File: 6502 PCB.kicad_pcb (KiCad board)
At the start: 2 copper layers, 25 parts, among them SW1 RESET, SW2 SW_Push, SW3 SW_Push, SW4 SW_Push, SW5 SW_Push, SW6 SW_Push, U1 W65C02S, U2 28C256, U3 62256, U4 W65C22, U5 74HC00, X1 1MHz

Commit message: bumb
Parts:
- DS1: footprint Display:HY1602E -> Display:WC1602A
- moved DS1 220.6 mm to (27.9, 87.9)
- moved U2 90.1 mm to (22.9, 53.3), turned to 90 degrees
- moved SW4 69.8 mm to (147.3, 104.1)
- moved SW1 68.2 mm to (27.9, 25.4)
- moved X1 65.9 mm to (63.5, 27.9)
- moved C4 64.3 mm to (125.5, 37.9)
- moved C2 64.3 mm to (125.5, 28.2)
- moved C3 64.3 mm to (125.5, 33.0)
- moved R1 64.3 mm to (130.1, 29.8)
- moved R2 64.3 mm to (130.1, 31.6)
- moved R3 64.3 mm to (130.1, 33.3)
- moved R4 64.3 mm to (130.1, 35.1)
- moved R5 64.3 mm to (130.1, 36.8)
- moved R6 64.3 mm to (130.1, 38.6)
- moved R7 64.3 mm to (130.1, 40.3)
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
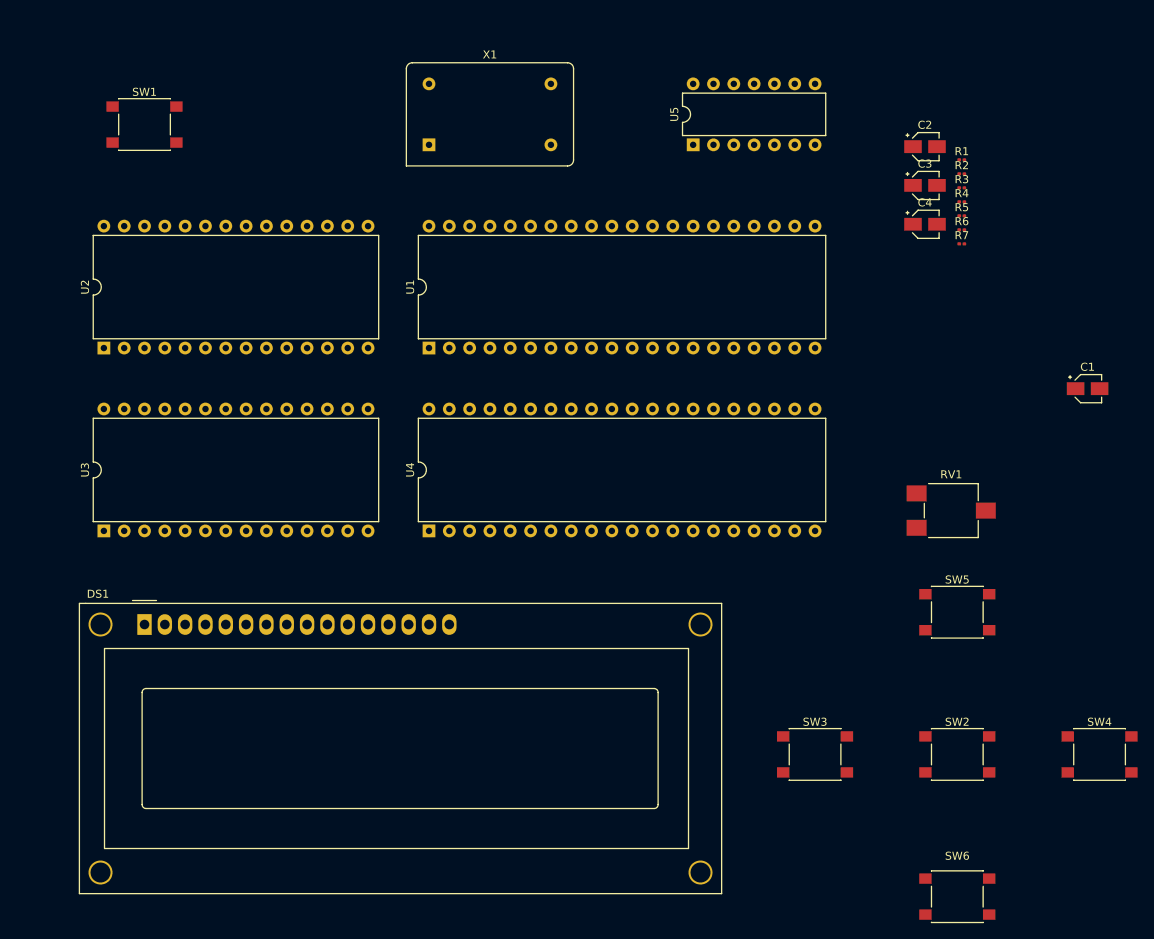
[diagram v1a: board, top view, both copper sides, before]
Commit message: Add files via upload
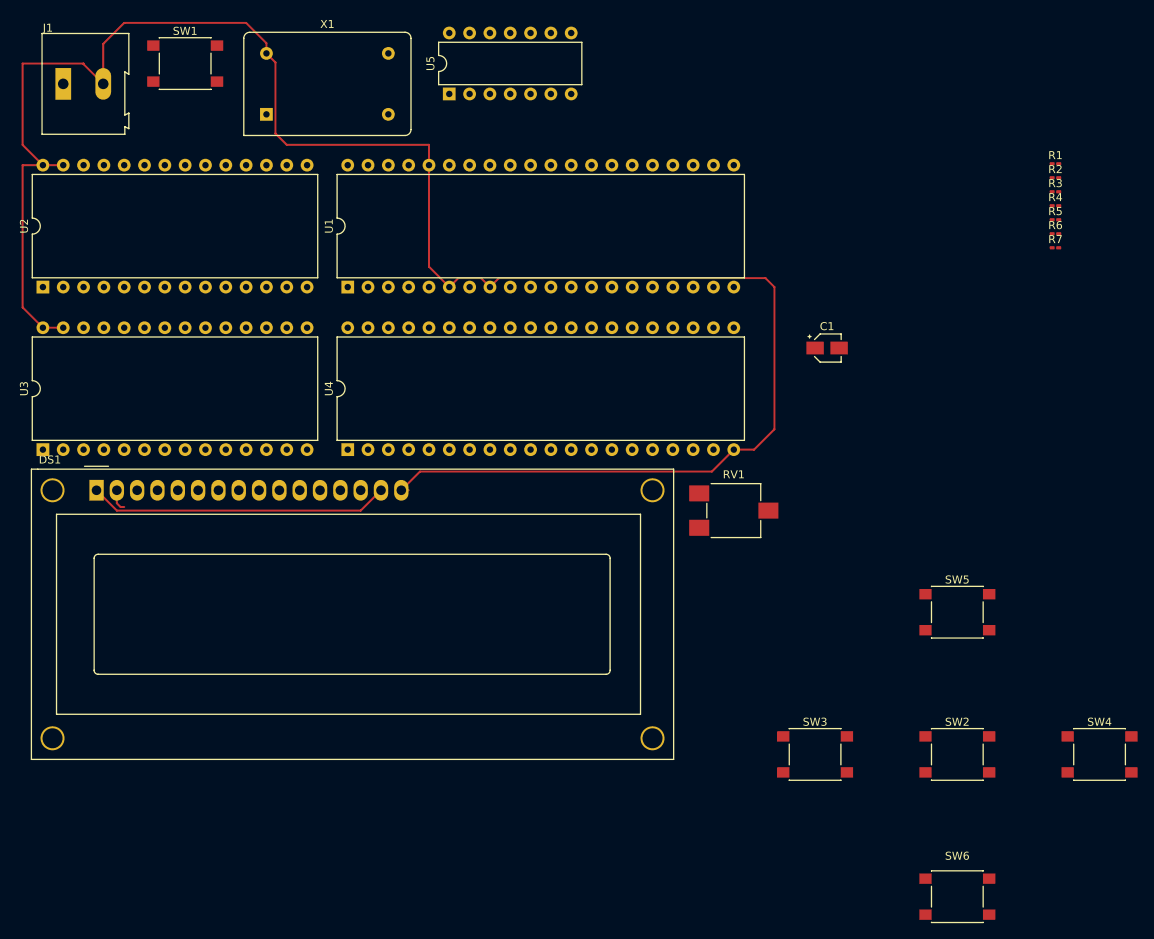
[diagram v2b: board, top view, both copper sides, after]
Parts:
- removed C2, C3, C4: 0.1uf, Capacitor_SMD:CP_Elec_3x5.3
- added J1: power_source, TerminalBlock:TerminalBlock_Altech_AK300-2_P5.00mm, F.Cu at (17.8, 20.3)
- DS1: value HY1602E -> HD44780U
- R1, R2, R3, R4, R5, R6, R7: footprint Resistor_SMD:R_0201_0603Metric -> Resistor_SMD:R_0201_0603Metric_Pad0.64x0.40mm_HandSolder
- moved C1 33.0 mm to (113.3, 53.3)
- moved U5 31.1 mm to (66.0, 21.6)
- moved RV1 27.2 mm to (101.6, 73.7)
- moved X1 20.7 mm to (43.2, 24.1)
- moved DS1 17.8 mm to (21.9, 71.1)
- moved U4 14.4 mm to (53.3, 66.0)
- moved U1 12.7 mm to (53.3, 45.7)
- moved U3 12.7 mm to (15.2, 66.0)
- moved R1 11.7 mm to (141.8, 30.3)
- moved R2 11.7 mm to (141.8, 32.1)
- moved R3 11.7 mm to (141.8, 33.8)
- moved R4 11.7 mm to (141.8, 35.6)
- moved R5 11.7 mm to (141.8, 37.3)
- moved R6 11.7 mm to (141.8, 39.1)
- moved R7 11.7 mm to (141.8, 40.8)
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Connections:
- C1 pad 2: GND -> /GND
- DS1 pad 1: GND -> /GND
- DS1 pad 15: GND -> /GND
- DS1 pad 16: +5V -> /VDD
- DS1 pad 2: +5V -> /VDD
- R1 pad 1: +5V -> /VDD
- R2 pad 1: +5V -> /VDD
- R3 pad 1: +5V -> Net-(U4-PA0)
- R3 pad 2: Net-(U4-PA0) -> /VDD
- R4 pad 1: +5V -> Net-(U4-PA1)
- R4 pad 2: Net-(U4-PA1) -> /VDD
- R5 pad 1: +5V -> Net-(U4-PA2)
- R5 pad 2: Net-(U4-PA2) -> /VDD
- R6 pad 1: +5V -> Net-(U4-PA3)
- R6 pad 2: Net-(U4-PA3) -> /VDD
- R7 pad 1: +5V -> Net-(U4-PA4)
- R7 pad 2: Net-(U4-PA4) -> /VDD
- RV1 pad 1: GND -> /GND
- SW1 pad 1: GND -> Net-(U1-~{RES})
- SW1 pad 2: Net-(U1-~{RES}) -> /GND
- SW2 pad 2: GND -> /GND
- SW3 pad 2: GND -> /GND
- SW4 pad 2: GND -> /GND
- SW5 pad 2: GND -> /GND
- SW6 pad 2: GND -> /GND
- U1 pad 21: GND -> /GND
- U1 pad 36: +5V -> /VDD
- U1 pad 6: +5V -> /VDD
- U1 pad 8: +5V -> /VDD
- U2 pad 14: GND -> /GND
- U2 pad 22: GND -> /GND
- U2 pad 27: +5V -> /VDD
- U2 pad 28: +5V -> /VDD
- U3 pad 14: GND -> /GND
- U3 pad 22: GND -> /GND
- U3 pad 27: +5V -> /VDD
- U3 pad 28: +5V -> /VDD
- U4 pad 1: GND -> /GND
- U4 pad 20: +5V -> /VDD
- X1 pad 14: +5V -> /VDD
- X1 pad 7: GND -> /GND
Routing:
- net /VDD: track 0.00 -> 245.6 mm
- net /GND: track 0.00 -> 37.7 mm

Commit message: Add files via upload
almost done with pcb design
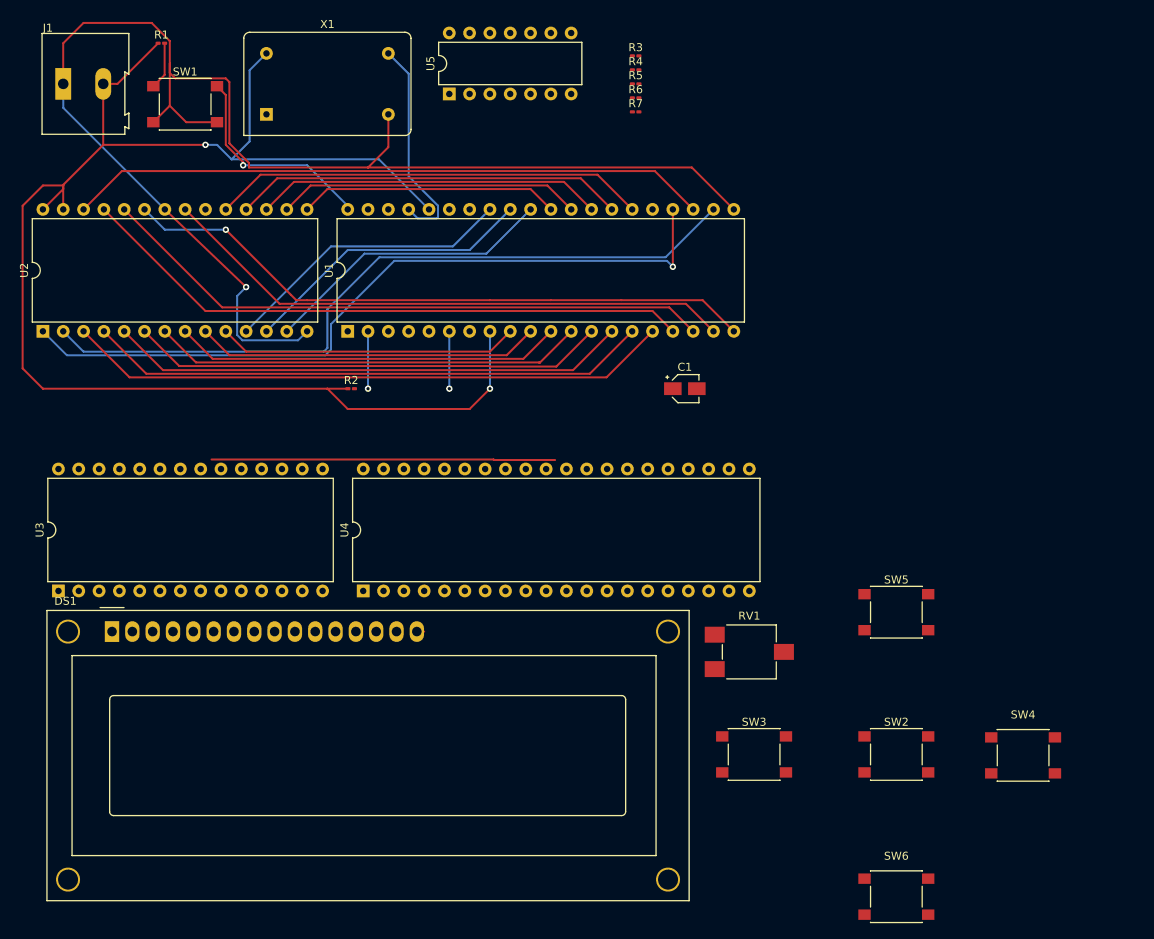
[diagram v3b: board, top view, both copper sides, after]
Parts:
- moved R1 112.8 mm to (30.0, 15.2)
- moved R2 91.9 mm to (53.8, 58.4)
- moved R3 55.2 mm to (89.3, 16.8)
- moved R4 55.2 mm to (89.3, 18.6)
- moved R5 55.2 mm to (89.3, 20.3)
- moved R6 55.2 mm to (89.3, 22.1)
- moved R7 55.2 mm to (89.3, 23.8)
- moved C1 18.5 mm to (95.5, 58.4)
- moved RV1 17.8 mm to (103.5, 91.3)
- moved DS1 17.8 mm to (23.9, 88.8)
- moved U3 17.8 mm to (17.2, 83.7)
- moved U4 17.8 mm to (55.3, 83.7)
- moved SW4 9.56 mm to (137.8, 104.3)
- moved SW3 7.62 mm to (104.1, 104.1)
- moved SW2 7.62 mm to (121.9, 104.1)
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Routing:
- net /GND: track 37.7 -> 180.4 mm, vias 0 -> 1
- net /a3: track 0.00 -> 97.1 mm
- net /a14: track 0.00 -> 94.2 mm, vias 0 -> 1
- net /a12: track 0.00 -> 92.5 mm
- net /a13: track 0.00 -> 80.2 mm
- net /a11: track 0.00 -> 80.0 mm, vias 0 -> 1
- net /a9: track 0.00 -> 77.4 mm
- net /a8: track 0.00 -> 77.4 mm
- net /a7: track 0.00 -> 75.9 mm
- net /a10: track 0.00 -> 72.4 mm
- net /a6: track 0.00 -> 70.4 mm
- net /a5: track 0.00 -> 65.0 mm
- net /a4: track 0.00 -> 59.5 mm
- net /d7: track 0.00 -> 54.4 mm
- net /VDD: track 245.6 -> 195.8 mm, vias 0 -> 3
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
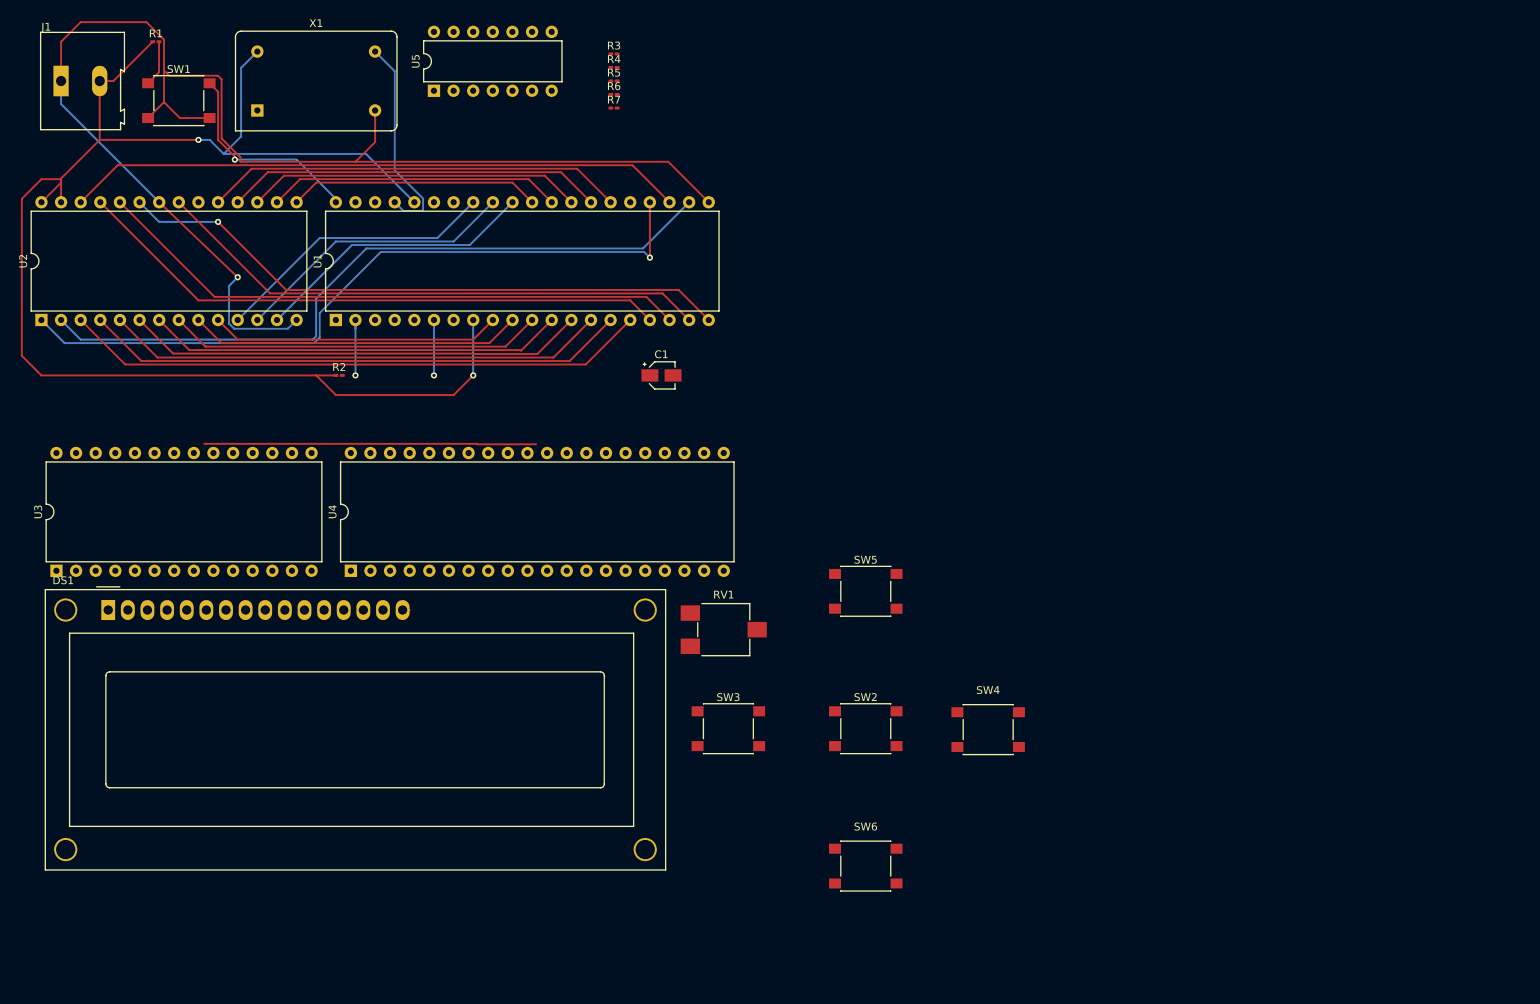
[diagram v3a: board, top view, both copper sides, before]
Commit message: Add files via upload
redid pretty much everything
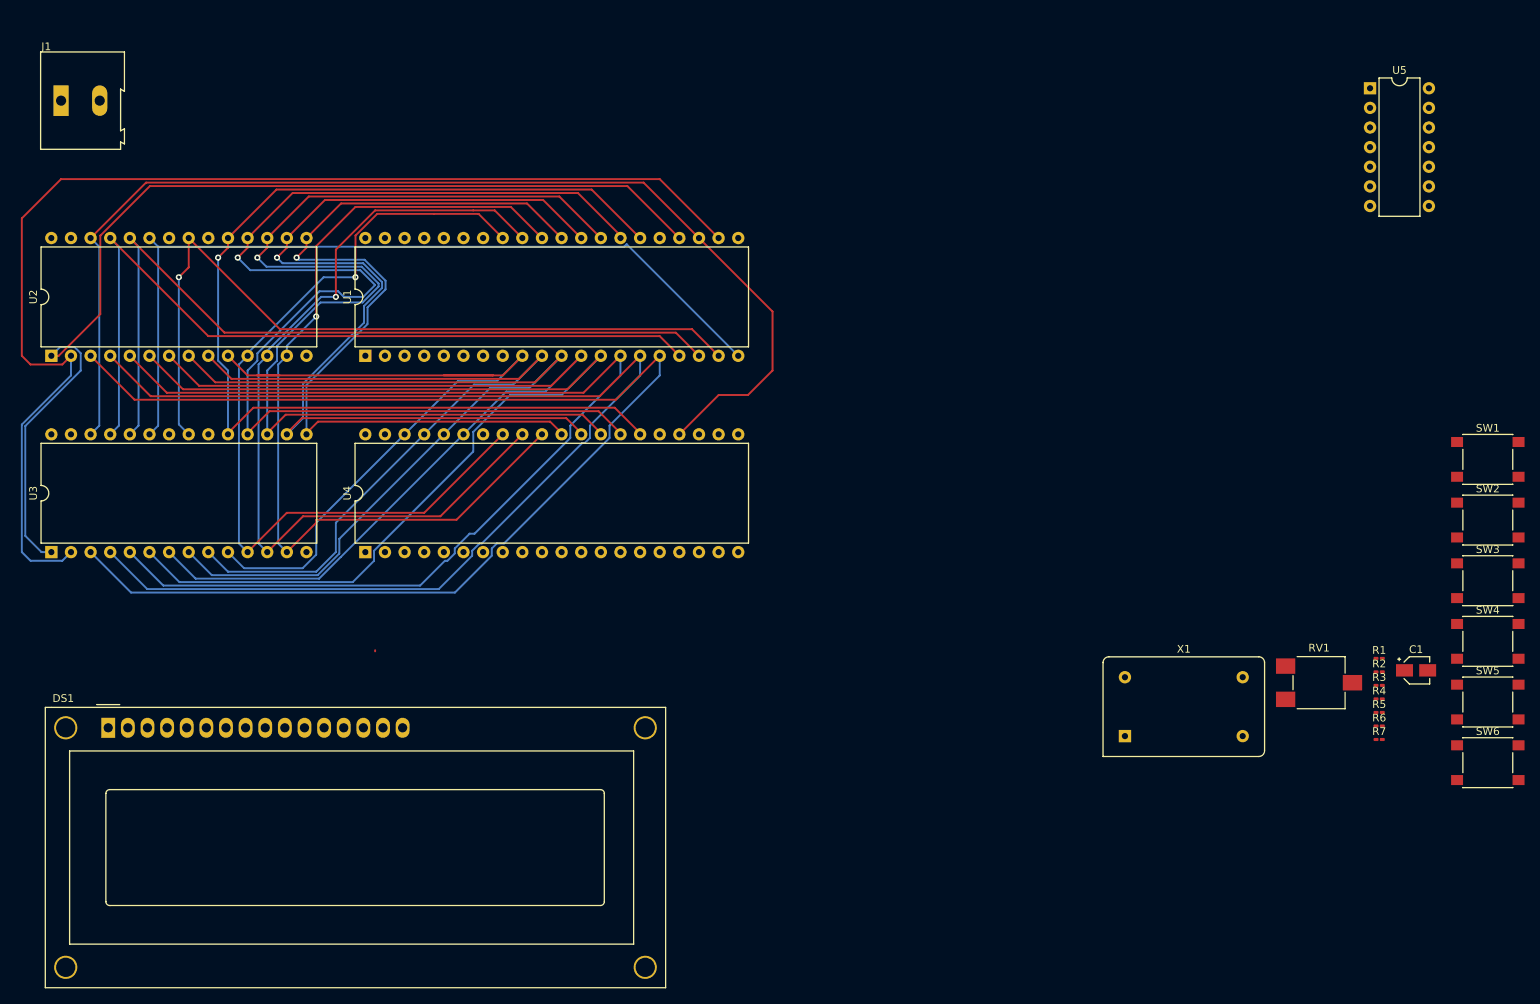
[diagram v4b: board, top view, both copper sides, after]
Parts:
- moved R1 177.3 mm to (188.4, 95.0)
- moved SW1 175.6 mm to (202.4, 69.3)
- moved R2 139.9 mm to (188.4, 96.8)
- moved X1 138.4 mm to (155.5, 105.1)
- moved R3 128.4 mm to (188.4, 98.5)
- moved R4 128.4 mm to (188.4, 100.3)
- moved R5 128.4 mm to (188.4, 102.0)
- moved R6 128.4 mm to (188.4, 103.8)
- moved R7 128.4 mm to (188.4, 105.5)
- moved U5 121.1 mm to (187.2, 21.3), turned to 0 degrees
- moved C1 104.9 mm to (193.1, 96.6)
- moved SW3 100.1 mm to (202.4, 85.0)
- moved SW2 84.9 mm to (202.4, 77.1)
- moved SW5 81.8 mm to (202.4, 100.7)
- moved SW6 81.6 mm to (202.4, 108.5)
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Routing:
- net /VDD: track 195.8 -> 0.00 mm, vias 3 -> 0
- net /GND: track 180.4 -> 0.15 mm, vias 1 -> 0
- net /d6: track 48.9 -> 156.7 mm, vias 0 -> 1
- net /d5: track 43.5 -> 141.6 mm, vias 0 -> 1
- net /a7: track 75.9 -> 169.8 mm
- net /a6: track 70.4 -> 158.8 mm
- net /d7: track 54.4 -> 141.1 mm, vias 0 -> 1
- net /d4: track 38.0 -> 124.7 mm, vias 0 -> 1
- net /a5: track 65.0 -> 147.9 mm
- net /d3: track 32.6 -> 110.9 mm, vias 0 -> 1
- net /d2: track 36.8 -> 114.6 mm, vias 0 -> 1
- net /a4: track 59.5 -> 136.4 mm
- net /d1: track 36.8 -> 111.9 mm, vias 0 -> 1
- net /d0: track 36.8 -> 110.9 mm, vias 0 -> 1
- net /a13: track 80.2 -> 147.6 mm
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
